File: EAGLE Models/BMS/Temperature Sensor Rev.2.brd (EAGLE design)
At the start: 160 x 100 mm, 9 parts, among them IC2 TL331

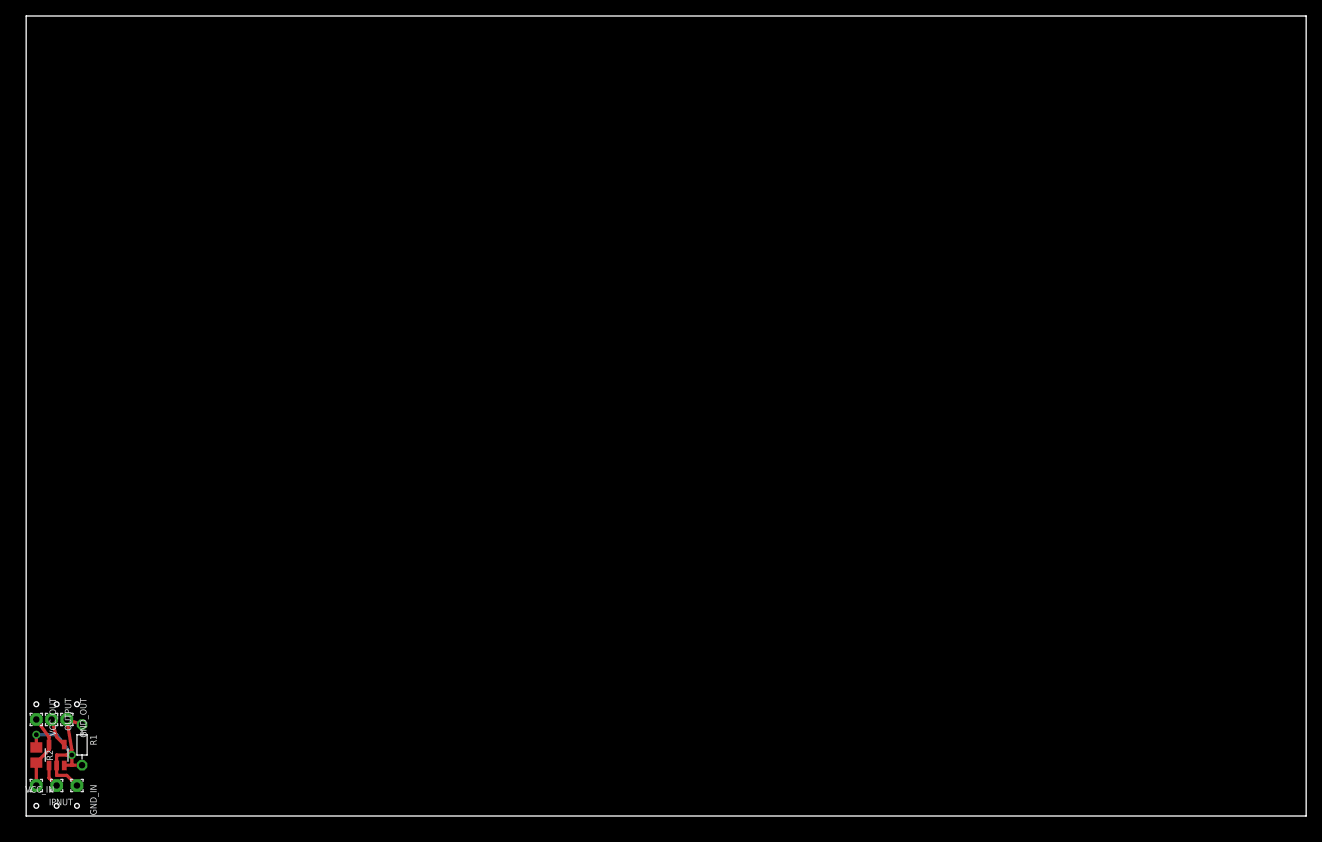
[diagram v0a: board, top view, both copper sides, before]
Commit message: Made an okboard layout
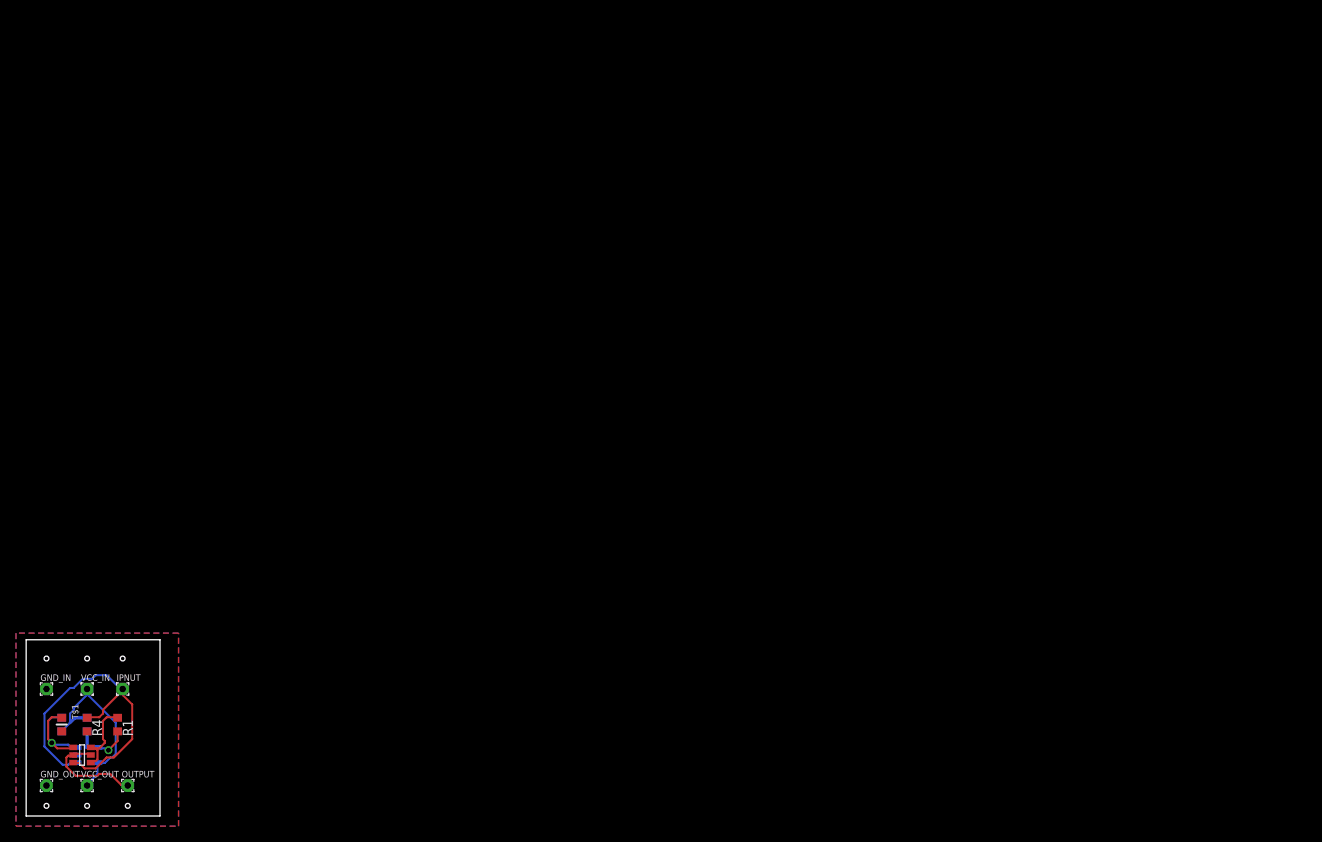
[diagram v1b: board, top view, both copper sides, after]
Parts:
- added R3, R4: (no value), resistor:R0603
- added T$1: THERMISTOR, formula electric:0603
- added _: DMG6602, formula electric:SOT23-6
- R1: value THERMISTOR-5 -> (none); device varistor:R-5 -> resistor:R0603
- R2: device resistor:R0805 -> resistor:R0603
- moved IPNUT 14.6 mm to (12.1, 15.9), turned to 0 degrees
- moved VCC_IN 13.6 mm to (7.62, 15.9), turned to 0 degrees
- moved GND_IN 12.7 mm to (2.54, 15.9)
- moved OUTPUT 12.6 mm to (12.7, 3.81), turned to 0 degrees
- moved VCC_OUT 10.4 mm to (7.62, 3.81)
- moved GND_OUT 8.64 mm to (2.54, 3.81)
- moved R1 5.12 mm to (11.4, 11.4)
- moved R2 4.96 mm to (4.45, 11.4), flipped to the bottom, turned to 90 degrees
- moved IC2 3.81 mm to (7.62, 7.62), flipped to the bottom, turned to 90 degrees
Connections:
- removed net N$1: IC2.3, R1.2, R2.1
- new net COMP_OUT: IC2.4, R1.2, R3.2
- new net MOS_IN: R1.1, _.P$1, _.P$3
- new net THERM_OUT: IC2.3, R2.2, T$1.P$1, _.P$4
- net GND: now also R4.2, T$1.P$2; no longer R1.1
- net INPUT: now also R4.1, _.P$6
- net OUTPUT: now also _.P$2, _.P$5; no longer IC2.4
- net VCC: now also R2.1, R3.1; no longer R2.2
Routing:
- net INPUT: track 2.90 -> 43.9 mm
- net THERM_OUT: track 0.00 -> 16.1 mm, vias 0 -> 1
- net VCC: track 9.42 -> 24.8 mm
- net GND: track 13.6 -> 0.00 mm
- net N$1: track 10.8 -> 0.00 mm, vias 2 -> 0
- net OUTPUT: track 3.62 -> 13.3 mm
- net MOS_IN: track 0.00 -> 9.47 mm
- net COMP_OUT: track 0.00 -> 7.83 mm, vias 0 -> 1
- added copper zone on layer 1, net GND
- added copper zone on layer 16, net GND
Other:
- board size 160 x 100 mm -> 16.7 x 22 mm
